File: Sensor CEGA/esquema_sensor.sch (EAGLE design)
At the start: 8 parts, among them J1 DCJ0202

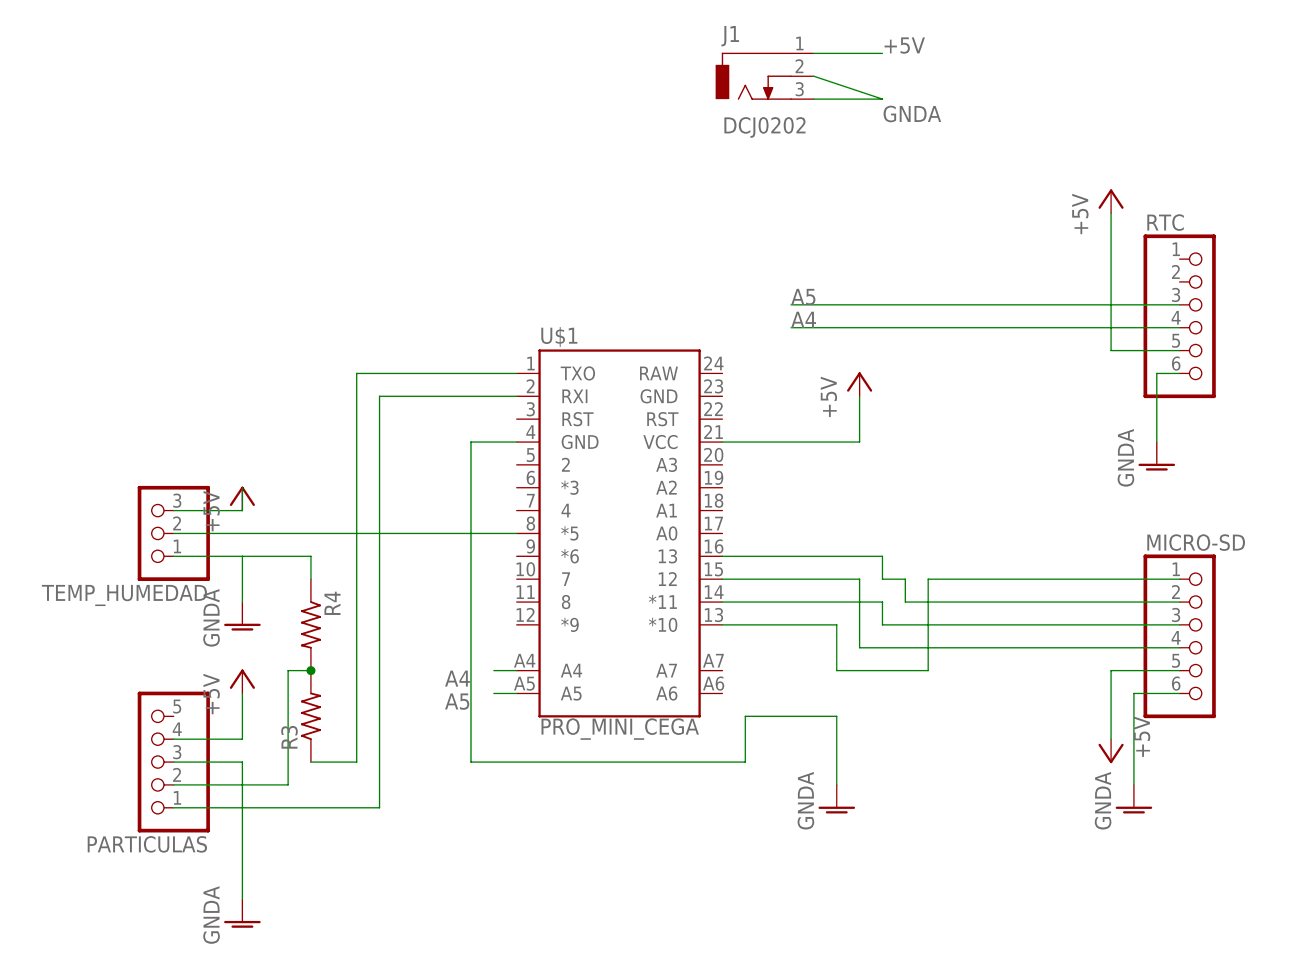
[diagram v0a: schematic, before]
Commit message: last version and fotos
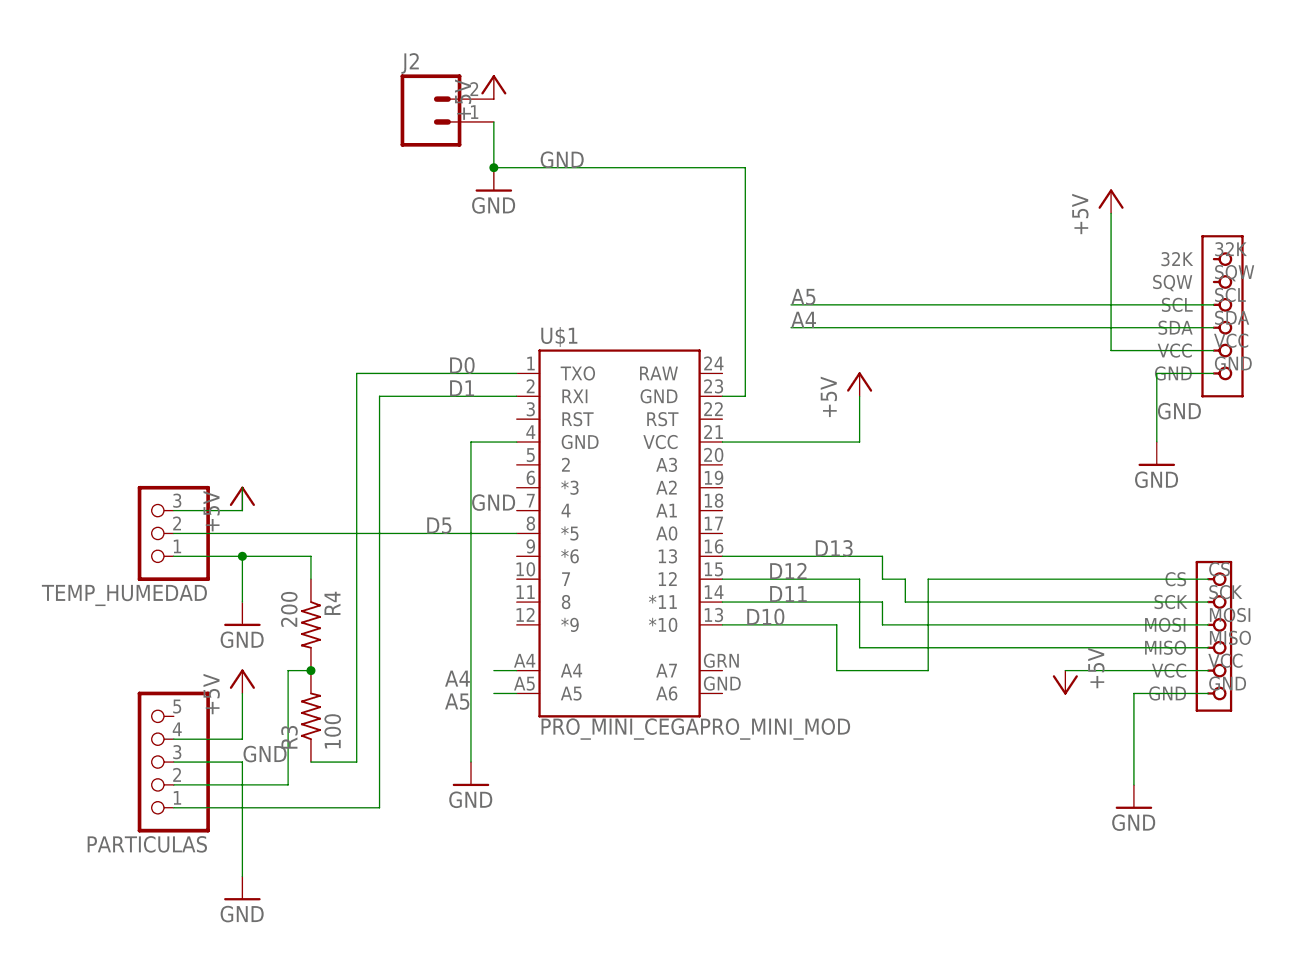
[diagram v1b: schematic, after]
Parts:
- removed J1: DCJ0202, con-jack:DCJ0202
- removed MICRO-SD: (no value), adafruit:PINHD-1X6B
- added J2: (no value), SparkFun-Connectors:M025MM
- added SD_READER: MICRO_SD_READER, fablab_uchile:MICRO_SD_READER
- R3: value (none) -> 100
- R4: value (none) -> 200
- RTC: value (none) -> DS3231_RTC; device adafruit:PINHD-1X6B -> fablab_uchile:DS3231_RTC
- U$1: value PRO_MINI_CEGA -> PRO_MINI_CEGAPRO_MINI_MOD; device fablab_uchile:PRO_MINI_CEGA -> fablab_uchile:PRO_MINI_CEGAPRO_MINI_MOD
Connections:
- net N$5 renamed D1
- net N$6 renamed D0
- net N$8 renamed D5
- removed net GNDA: J1.2, J1.3, MICRO-SD.6, PARTICULAS.3, R4.1, RTC.6, TEMP_HUMEDAD.1, U$1.GND
- removed net N$10: MICRO-SD.4, U$1.12
- removed net N$11: MICRO-SD.3, U$1.*11
- removed net N$12: MICRO-SD.2, U$1.13
- removed net N$13: MICRO-SD.1, U$1.*10
- new net D10: SD_READER.CS, U$1.*10
- new net D11: SD_READER.MOSI, U$1.*11
- new net D12: SD_READER.MISO, U$1.12
- new net D13: SD_READER.SCK, U$1.13
- new net GND: J2.1, PARTICULAS.3, R4.1, RTC.GND, SD_READER.GND, TEMP_HUMEDAD.1, U$1.GND, U$1.GND@2
- net +5V: now also J2.2, RTC.VCC, SD_READER.VCC; no longer J1.1, MICRO-SD.5, RTC.5
- net A4: now also RTC.SDA; no longer RTC.4
- net A5: now also RTC.SCL; no longer RTC.3
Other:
- moved on the sheet: U$1
